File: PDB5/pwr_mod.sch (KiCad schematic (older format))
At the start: 10 parts, among them Q1 BC847CE6327HTSA1, U11 74LVC1G08, U12 AUIPS7111S

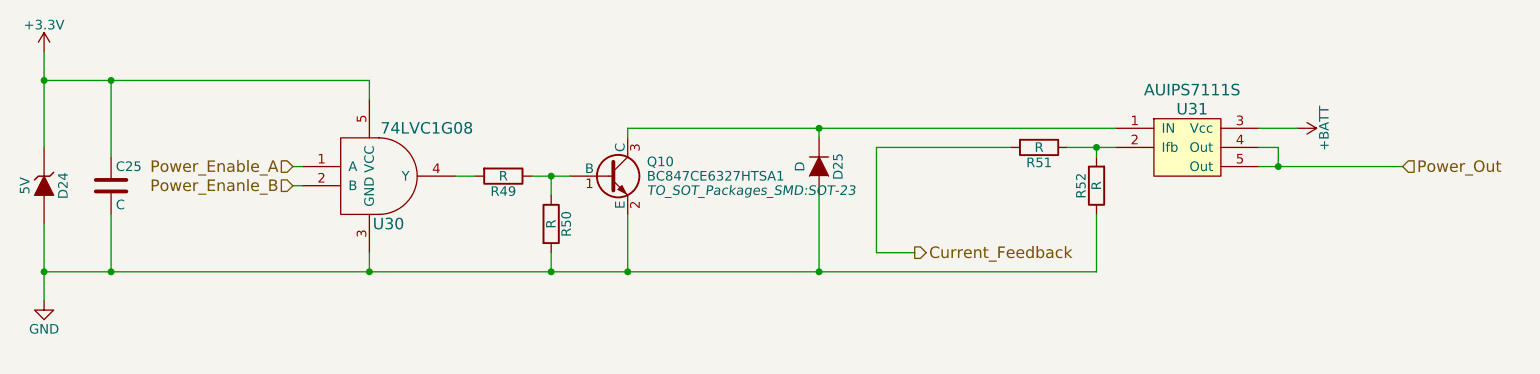
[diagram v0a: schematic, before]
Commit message: test
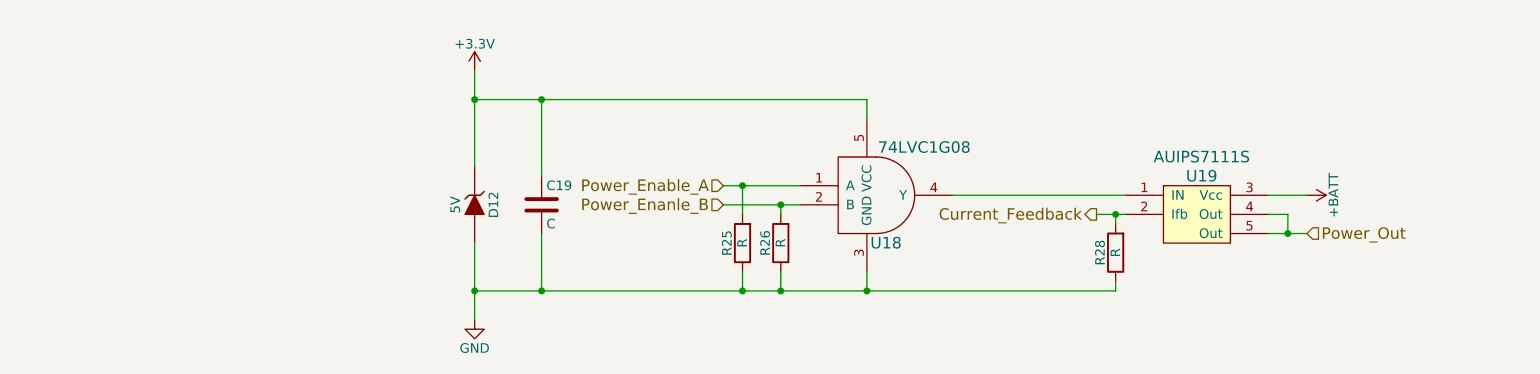
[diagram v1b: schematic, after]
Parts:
- removed D6: D, Diodes_SMD:D_0603, symbol D
- removed Q1: BC847CE6327HTSA1, TO_SOT_Packages_SMD:SOT-23, symbol BC847CE6327HTSA1
- removed R5, R6: R, Resistors_SMD:R_0603, symbol R
- added R26: R, Resistors_SMD:R_0603, symbol R
- U12: footprint TO_SOT_Packages_SMD:TO-263-5Lead -> KiCad-Dev:TO-263-!3
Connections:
- net Current_Feedback: now also R7.2, U12.2 (Ifb)
- net GND: now also R4.1, R26.1
- net Power_Enable_A: now also R4.2
- net Power_Enanle_B: now also R26.2
- net at U12.1 (IN): now also U11.4 (Y)
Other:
- moved on the sheet: C19, D12, R28, U18, U19
